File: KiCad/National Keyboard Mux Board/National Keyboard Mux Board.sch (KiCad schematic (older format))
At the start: 43 parts, among them J1 Conn_01x01_Female, J10 Conn_01x01_Female, J11 Conn_01x01_Female, J12 Conn_01x01_Female, J13 Conn_01x01_Female, J14 Conn_01x01_Female, J15 Conn_01x01_Female, J16 Conn_01x01_Female, J17 Conn_01x01_Female, J18 Conn_01x01_Female, J19 Conn_02x08_Odd_Even, J2 Conn_01x01_Female, J3 Conn_01x01_Female, J4 Conn_01x01_Female, J5 Conn_01x01_Female, J6 Conn_01x01_Female, J7 Conn_01x01_Female, J8 Conn_01x01_Female, J9 Conn_01x01_Female

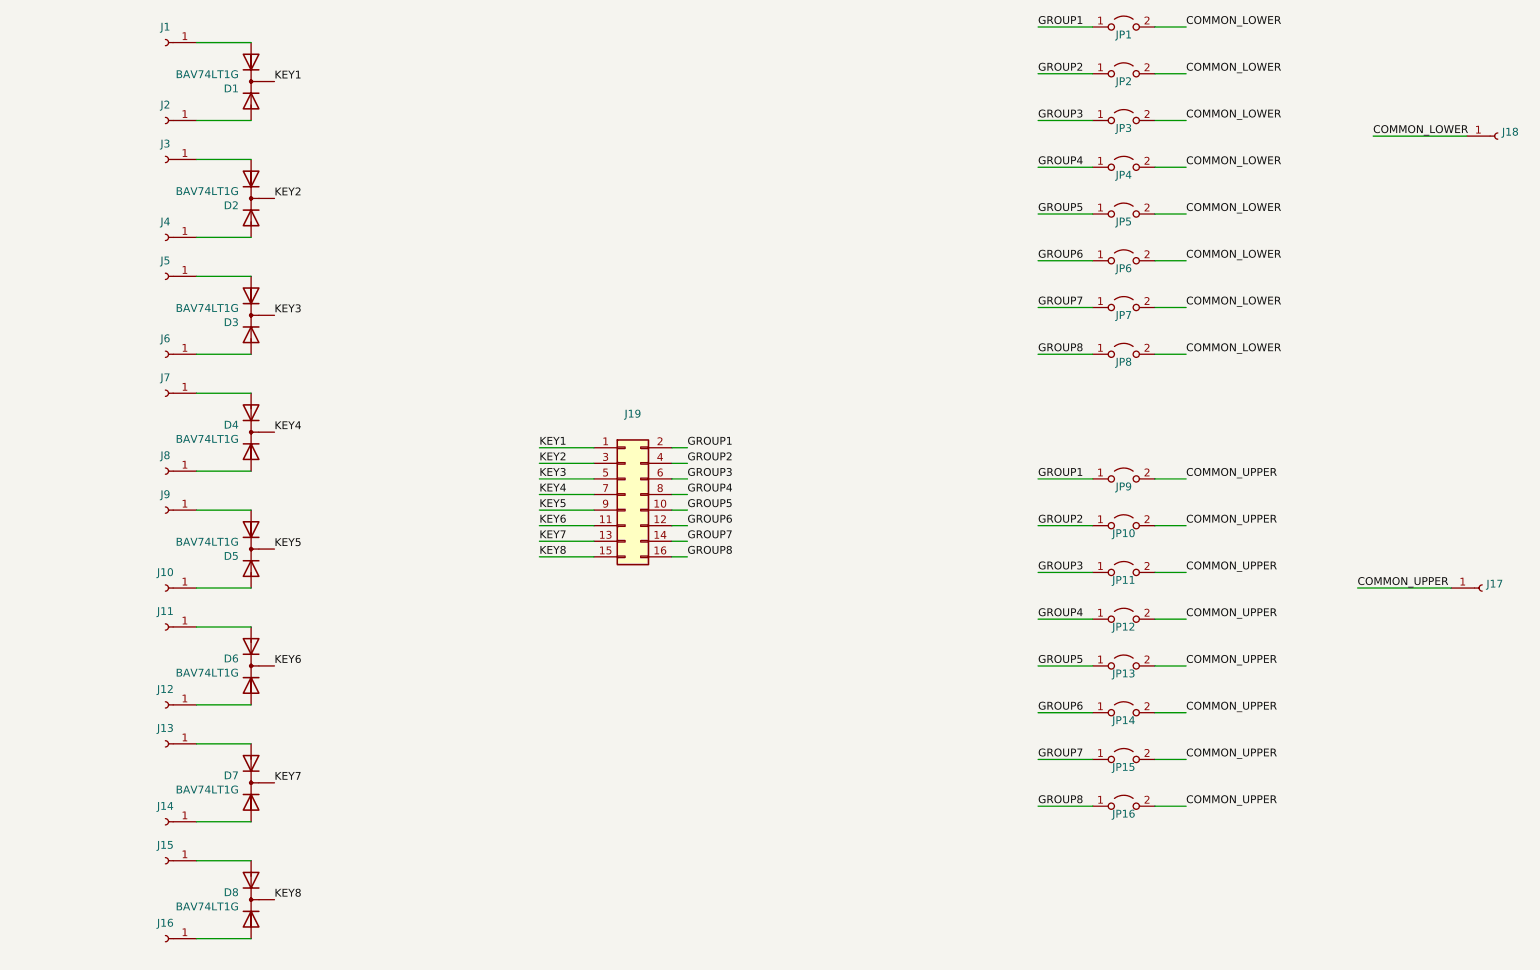
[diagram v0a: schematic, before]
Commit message: production files
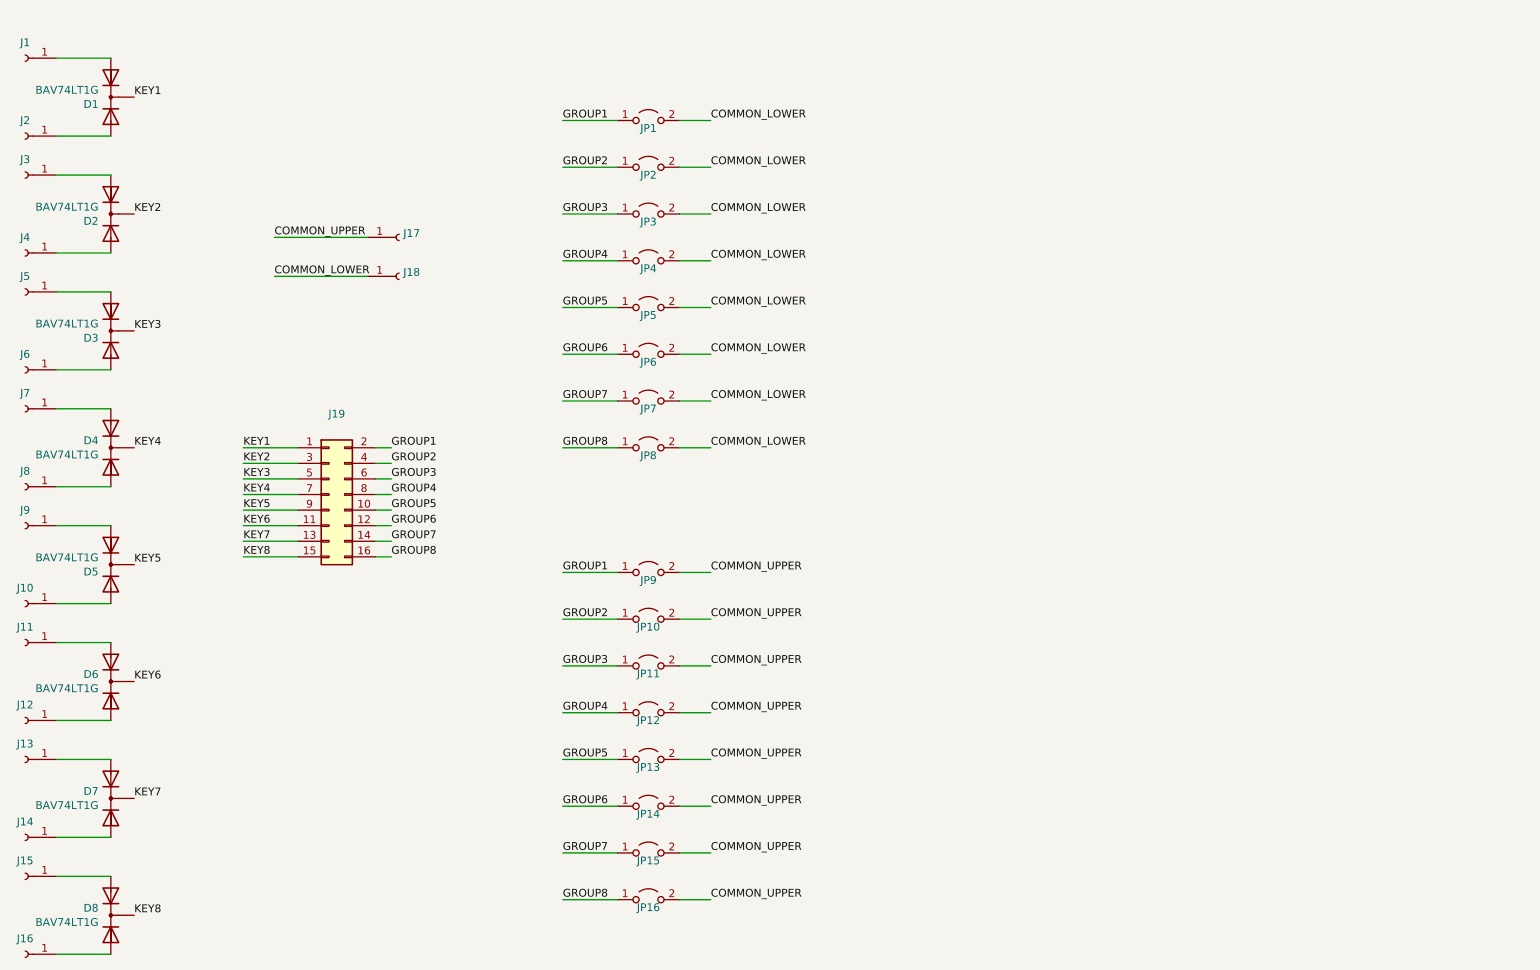
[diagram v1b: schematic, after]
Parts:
- D1, D2, D3, D4, D5, D6, D7, D8: LCSC (none) -> C82481
- J19: LCSC (none) -> C492443
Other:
- moved on the sheet: D1, D2, D3, D4, D5, D6, D7, D8, J1, J10, J11, J12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
